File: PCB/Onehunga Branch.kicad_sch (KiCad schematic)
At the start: 5 parts

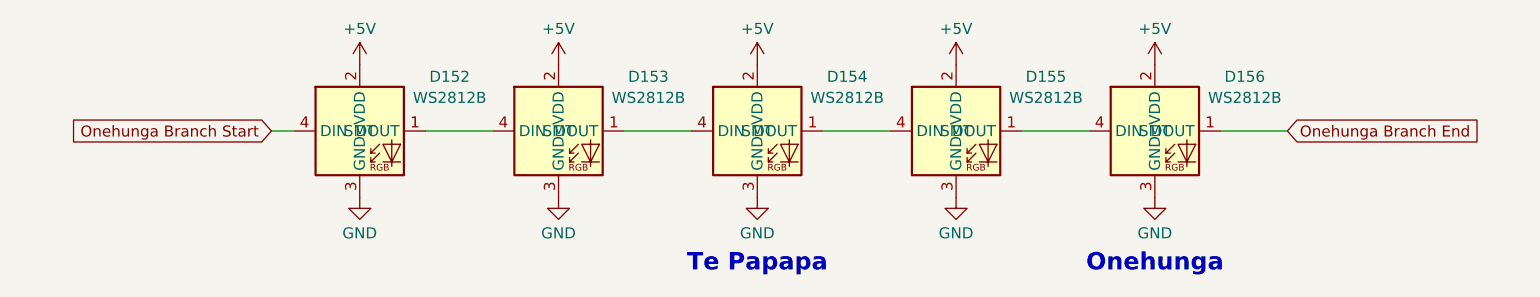
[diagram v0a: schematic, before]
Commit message: V1.1.0 PCB
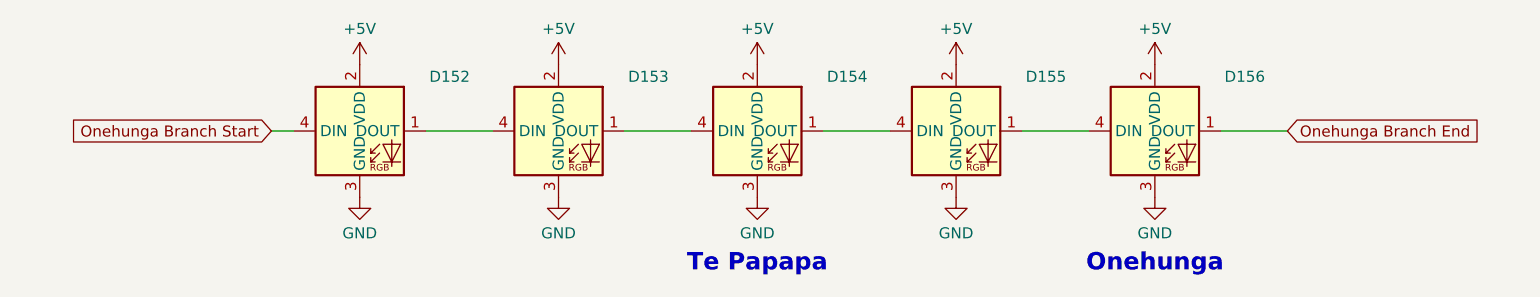
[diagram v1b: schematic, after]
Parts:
- D152, D153, D154, D155, D156: value WS2812B -> XL-1615RGBC-WS2812B-S; LCSC C5349954 -> C41413180; Manufacturer XINGLIGHT -> (none); Part XL-1615RGBC-WS2812B -> (none); Process SMT -> (none)
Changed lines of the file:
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@@
 	(title_block
 		(title "Auckland Train Network Live Map")
-		(date "2025-04-26")
-		(rev "1")
+		(date "2025-06-23")
+		(rev "1.1.0")
 		(company "Kea Studios")
 		(comment 1 "©Chris Dirks")
@@
 			)
 		)
-		(property "Value" "WS2812B"
+		(property "Value" "XL-1615RGBC-WS2812B-S"
 			(at 104.3176 21.5777 0)
 			(effects
@@
 					(size 1.27 1.27)
 				)
+				(hide yes)
 			)
 		)
@@
 			)
 		)
-		(property "LCSC" "C5349954"
+		(property "LCSC" "C41413180"
 			(at 93.98 25.4 0)
 			(effects
@@
 			)
 		)
-		(property "Part" "XL-1615RGBC-WS2812B"
+		(property "Circuits" ""
 			(at 93.98 25.4 0)
 			(effects
@@
 			)
 		)
-		(property "Manufacturer" "XINGLIGHT"
+		(property "Current Rating" ""
 			(at 93.98 25.4 0)
 			(effects
@@
 			)
 		)
-		(property "PartID" ""
+		(property "DC Resistance" ""
 			(at 93.98 25.4 0)
 			(effects
@@
 					(size 1.27 1.27)
 				)
-			)
-		)
-		(property "Process" "SMT"
+				(hide yes)
+			)
+		)
+		(property "Impedance @ Frequency" ""
 			(at 93.98 25.4 0)
 			(effects
@@
 					(size 1.27 1.27)
 				)
+				(hide yes)
 			)
 		)
@@
 			)
 		)
-		(property "Value" "WS2812B"
+		(property "Value" "XL-1615RGBC-WS2812B-S"
 			(at 58.5976 21.5777 0)
 			(effects
@@
 					(size 1.27 1.27)
 				)
+				(hide yes)
 			)
 		)
@@
 			)
 		)
-		(property "LCSC" "C5349954"
+		(property "LCSC" "C41413180"
 			(at 48.26 25.4 0)
 			(effects
@@
 			)
 		)
-		(property "Part" "XL-1615RGBC-WS2812B"
+		(property "Circuits" ""
 			(at 48.26 25.4 0)
 			(effects
@@
 			)
 		)
-		(property "Manufacturer" "XINGLIGHT"
+		(property "Current Rating" ""
 			(at 48.26 25.4 0)
 			(effects
@@
 			)
 		)
-		(property "PartID" ""
+		(property "DC Resistance" ""
 			(at 48.26 25.4 0)
 			(effects
@@
 					(size 1.27 1.27)
 				)
-			)
-		)
-		(property "Process" "SMT"
+				(hide yes)
+			)
+		)
+		(property "Impedance @ Frequency" ""
 			(at 48.26 25.4 0)
 			(effects
@@
 					(size 1.27 1.27)
 				)
+				(hide yes)
 			)
 		)
@@
 			)
 		)
-		(property "Value" "WS2812B"
+		(property "Value" "XL-1615RGBC-WS2812B-S"
 			(at 150.0376 21.5777 0)
 			(effects
@@
 					(size 1.27 1.27)
 				)
+				(hide yes)
 			)
 		)
@@
 			)
 		)
-		(property "LCSC" "C5349954"
+		(property "LCSC" "C41413180"
 			(at 139.7 25.4 0)
 			(effects
@@
 			)
 		)
-		(property "Part" "XL-1615RGBC-WS2812B"
+		(property "Circuits" ""
 			(at 139.7 25.4 0)
 			(effects
@@
 			)
 		)
-		(property "Manufacturer" "XINGLIGHT"
+		(property "Current Rating" ""
 			(at 139.7 25.4 0)
 			(effects
@@
 			)
 		)
-		(property "PartID" ""
+		(property "DC Resistance" ""
 			(at 139.7 25.4 0)
 			(effects
@@
 					(size 1.27 1.27)
 				)
-			)
-		)
-		(property "Process" "SMT"
+				(hide yes)
+			)
+		)
+		(property "Impedance @ Frequency" ""
 			(at 139.7 25.4 0)
 			(effects
@@
 					(size 1.27 1.27)
 				)
+				(hide yes)
 			)
 		)
@@
 			)
 		)
-		(property "Value" "WS2812B"
+		(property "Value" "XL-1615RGBC-WS2812B-S"
 			(at 81.4576 21.5777 0)
 			(effects
@@
 					(size 1.27 1.27)
 				)
+				(hide yes)
 			)
 		)
@@
 			)
 		)
-		(property "LCSC" "C5349954"
+		(property "LCSC" "C41413180"
 			(at 71.12 25.4 0)
 			(effects
@@
 			)
 		)
-		(property "Part" "XL-1615RGBC-WS2812B"
+		(property "Circuits" ""
 			(at 71.12 25.4 0)
 			(effects
@@
 			)
 		)
-		(property "Manufacturer" "XINGLIGHT"
+		(property "Current Rating" ""
 			(at 71.12 25.4 0)
 			(effects
@@
 			)
 		)
-		(property "PartID" ""
+		(property "DC Resistance" ""
 			(at 71.12 25.4 0)
 			(effects
@@
 					(size 1.27 1.27)
 				)
-			)
-		)
-		(property "Process" "SMT"
+				(hide yes)
+			)
+		)
+		(property "Impedance @ Frequency" ""
 			(at 71.12 25.4 0)
 			(effects
@@
 					(size 1.27 1.27)
 				)
+				(hide yes)
 			)
 		)
@@
 			)
 		)
-		(property "Value" "WS2812B"
+		(property "Value" "XL-1615RGBC-WS2812B-S"
 			(at 127.1776 21.5777 0)
 			(effects
@@
 					(size 1.27 1.27)
 				)
+				(hide yes)
 			)
 		)
@@
 			)
 		)
-		(property "LCSC" "C5349954"
+		(property "LCSC" "C41413180"
 			(at 116.84 25.4 0)
 			(effects
@@
 			)
 		)
-		(property "Part" "XL-1615RGBC-WS2812B"
+		(property "Circuits" ""
 			(at 116.84 25.4 0)
 			(effects
@@
 			)
 		)
-		(property "Manufacturer" "XINGLIGHT"
+		(property "Current Rating" ""
 			(at 116.84 25.4 0)
 			(effects
@@
 			)
 		)
-		(property "PartID" ""
+		(property "DC Resistance" ""
 			(at 116.84 25.4 0)
 			(effects
@@
 					(size 1.27 1.27)
 				)
-			)
-		)
-		(property "Process" "SMT"
+				(hide yes)
+			)
+		)
+		(property "Impedance @ Frequency" ""
 			(at 116.84 25.4 0)
 			(effects
@@
 					(size 1.27 1.27)
 				)
-			)
-		)
+				(hide yes)
+			)
+		)
